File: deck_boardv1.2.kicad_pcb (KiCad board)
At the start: 2 copper layers, 146.7 x 69.5 mm, 58 parts, among them Q1 Q_PMOS_GSD, Q2 Q_PMOS_GSD, Q3 NMOS, Q4 Q_PI, Q5 TIP122, Q6 Q_NPN_BEC, SW1 SAFE_switch, SW3 SAFE_switch, U1 Raspberry Pi Zero 2 W, U2 LT8610AC, U3 XBP24-Z7SIT-004, U4 ADP7158ARDZ-3.3-R7

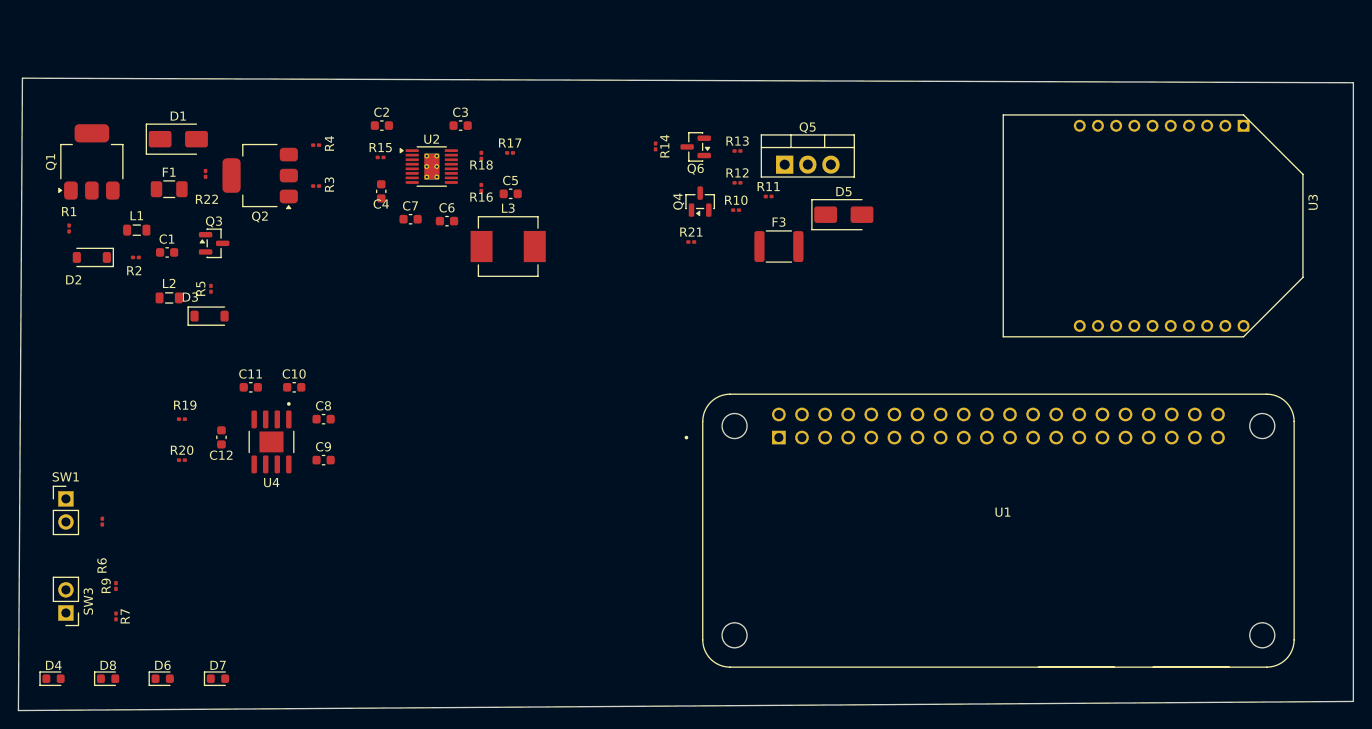
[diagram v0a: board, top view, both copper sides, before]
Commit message: PCB is mostly laid out, routing is WIP
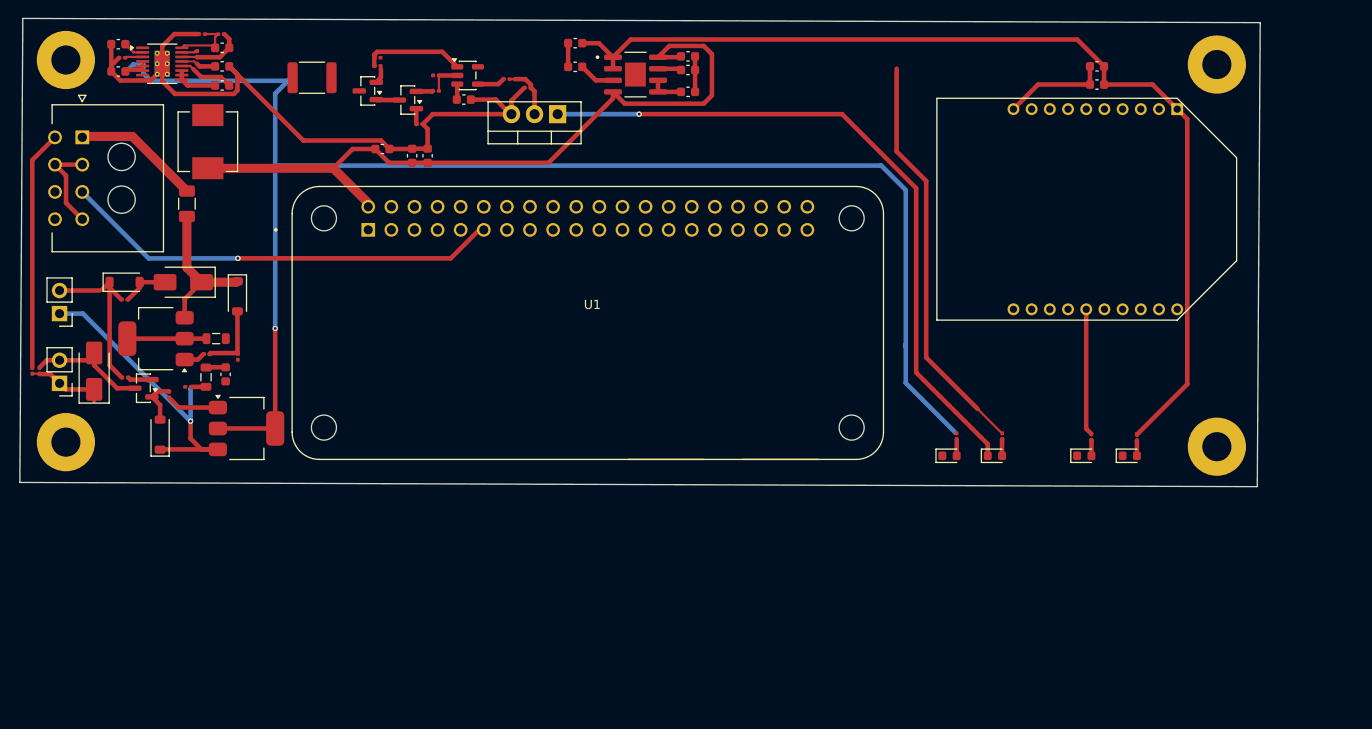
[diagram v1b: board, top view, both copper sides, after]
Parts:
- removed F3: Fuse, Fuse:Fuse_1812_4532Metric
- added ?: , , F.Cu at (187.0, 95.5)
- added ?: , , F.Cu at (187.0, 53.5)
- added ?: , , F.Cu at (60.5, 53.0)
- added ?: , , F.Cu at (60.5, 95.0)
- added C13: 0.1 µF, Capacitor_SMD:C_0603_1608Metric, F.Cu at (104.2, 57.4)
- added C14: 47µF, Capacitor_SMD:C_0603_1608Metric, F.Cu at (98.5, 63.5)
- added C15: 47pF, Capacitor_SMD:C_0603_1608Metric, F.Cu at (173.8, 55.7)
- added C16: 1µF, Capacitor_SMD:C_0603_1608Metric, F.Cu at (173.8, 53.7)
- added C17: 47µF, Capacitor_SMD:C_0603_1608Metric, F.Cu at (95.3, 62.8)
- added D9: BZT52B12, Diode_SMD:D_SOD-123, F.Cu at (67.0, 77.4)
- added F2: 1.0 A, Fuse:Fuse_1812_4532Metric, F.Cu at (87.5, 55.0)
- added J1: 430450800, HarnessDeck:MOLEX_430450800, F.Cu at (62.3, 61.5)
- added R23: 100kΩ, Resistor_SMD:R_0201_0603Metric, F.Cu at (57.6, 87.2)
- added R8: 100kΩ, Resistor_SMD:R_0201_0603Metric, F.Cu at (101.2, 54.7)
- added U5: 74LVC1G08, Package_TO_SOT_SMD:SOT-23-5, F.Cu at (104.7, 54.7)
- C1: value C -> 22 µF
- C7: value 100µF -> 47µF
- D1: value SMAJ33A -> SMAJ36A
- D2, D3: value D_Zener -> BZT52B12
- D5: value SMAJ33A -> 3.6 V Zener
- F1: value Fuse -> 045101.5
- L1, L2: value L -> 2.2µH
- L3: value 10µH -> 4.7µH
- Q1, Q2: value Q_PMOS_GSD -> FQPF27P06
- Q3: value NMOS -> 2N7000
- Q5: value TIP122 -> NMOS
- R1, R3: value 100 ohm -> 100Ω
- R10: value R -> 47Ω
- R11, R9: value R -> 100kΩ
- R15: value 110k -> 60.4kΩ
- R16: value 191k -> 100kΩ
- R17: value 1M -> 412kΩ
- R18: value 100k -> 100kΩ
- R19: value 1 kohm -> 1 kΩ
- R2, R4, R6: value 100 kohm -> 100kΩ
- R20: value 4.7/10 kohm -> 10 kΩ
- R21, R22: value 10 kohm -> 10kΩ
- R5: value 1 kohm -> 10kΩ
- R7: value R -> 10kΩ
- U3: value XBP24-Z7SIT-004 -> DIGI XBee-PRO 900HP RF Module (S3B)
- U4: value ADP7158ARDZ-3.3-R7 -> ADP7159
- moved D8 110.0 mm to (172.4, 96.5)
- moved D6 109.1 mm to (177.4, 96.5)
- moved R19 105.0 mm to (178.2, 94.5), turned to 90 degrees
- moved D4 101.5 mm to (157.6, 96.5)
- moved R20 100.0 mm to (173.2, 94.4), turned to 90 degrees
- moved D7 88.8 mm to (162.6, 96.5)
- moved R22 87.4 mm to (158.4, 94.4)
- moved D5 84.2 mm to (63.6, 87.2), turned to 90 degrees
- moved C12 66.2 mm to (128.9, 52.6), turned to 180 degrees
- moved R9 64.8 mm to (94.8, 52.8), turned to 0 degrees
- moved C9 56.9 mm to (128.9, 56.5), turned to 180 degrees
- moved U4 56.8 mm to (123.1, 54.6), turned to 0 degrees
- moved C10 55.6 mm to (128.9, 54.1), turned to 180 degrees
- moved U1 50.6 mm to (117.9, 81.9)
- moved C11 50.1 mm to (116.5, 53.8)
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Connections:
- C1 pad 2: /28v_inhibit/GND -> GND
- C5 pad 2: GND -> Net-(U2-FB)
- D1 pad 2: /28v_inhibit/GND -> GND
- D4 pad 1: /28v_inhibit/GND -> GND
- D5 pad 1: /28v_inhibit/28V_Post_Inhibit -> /Burn-Wire Circuit/ENABLE
- D5 pad 2: Net-(D5-A2) -> GND
- D7 pad 1: GND -> Net-(D7-K)
- Q3 pad 3: /28v_inhibit/GND -> GND
- Q5 pad 1: Net-(Q4-C) -> Net-(D7-K)
- Q5 pad 2: Net-(D5-A2) -> Net-(Q5-G)
- R10 pad 1: Net-(Q4-C) -> Net-(Q5-G)
- R10 pad 2: 3V3 -> Net-(R10-Pad2)
- R11 pad 2: Net-(Q4-C) -> Net-(Q5-G)
- R16 pad 2: GND -> Net-(U2-FB)
- R17 pad 1: GND -> Net-(U2-FB)
- R2 pad 2: /28v_inhibit/GND -> GND
- R21 pad 1: Net-(D5-A2) -> Net-(R21-Pad1)
- R6 pad 1: /28v_inhibit/GND -> GND
- R7 pad 1: Net-(SW3-A) -> /Burn-Wire Circuit/ENABLE
- R9 pad 1: GND -> /Burn-Wire Circuit/CTRL_IN
- R9 pad 2: Net-(SW3-A) -> GND
- SW3 pad 1: Net-(SW3-A) -> /Burn-Wire Circuit/ENABLE
- SW3 pad 2: /Burn-Wire Circuit/ENABLE -> GND
- U1 pad 11: unconnected-(U1-GPIO17-Camera_Select-Pad11) -> TE_1
- U1 pad 6: unconnected-(U1-GND_6-Pad6) -> GND
- U2 pad 16: GND -> Net-(U2-FB)
- U3 pad 14: 3V3 -> GND
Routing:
- net /28v_inhibit/28V_Post_Inhibit: track 0.00 -> 167.9 mm, vias 0 -> 1
- net GND: track 0.00 -> 128.0 mm
- net 3V3: track 0.00 -> 111.0 mm
- net 5V_Pi: track 0.00 -> 88.1 mm
- net Net-(D7-K): track 0.00 -> 75.4 mm, vias 0 -> 1
- net TE_1: track 0.00 -> 48.6 mm, vias 0 -> 1
- net Net-(R21-Pad1): track 0.00 -> 44.9 mm
- net /28v_inhibit/POST_INHIB1: track 0.00 -> 36.4 mm, vias 0 -> 1
- net TE_2: track 0.00 -> 26.3 mm
- net Net-(D9-K): track 0.00 -> 19.1 mm
- net Net-(D1-A1): track 0.00 -> 16.5 mm
- net /28v_inhibit/28v_IN: track 0.00 -> 14.0 mm
- net Net-(U3-ASSOCIATE/AD5/DIO5): track 0.00 -> 13.9 mm
- net /Burn-Wire Circuit/ENABLE: track 0.00 -> 12.4 mm
- net /Burn-Wire Circuit/CTRL_IN: track 0.00 -> 12.1 mm
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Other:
- board size 146.7 x 69.5 mm -> 136.3 x 51.5 mm
- board text added: "${REFERENCE}"
- board text added: "connection to burn-resistor off board"
- board text removed: "Access to Raspberry Pi ports in case"
- board text removed: "Antenna goes here"
- board text removed: "Digi XBee-PRO Module"
- board text removed: "Inhibit 2"
- board text removed: "RBF pins for inhibits"
- board text removed: "SD card located here"
- board text removed: "buck for 28V"
- board text removed: "inhibit 1"
- board text removed: "voltage converter for RF module"
